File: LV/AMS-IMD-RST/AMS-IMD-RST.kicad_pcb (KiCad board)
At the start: 2 copper layers, 76.3 x 61.5 mm, 56 parts, among them J1 2P Droit 2-11-2022, J2 2P Droit 2-11-2022, J3 2P Droit 2-11-2022, J4 2P Droit 2-11-2022, J5 2P Droit 2-11-2022, J7 4P Droit 22-11-2042, K1 Relais PCB, K2 Bistable V23079B1201B301, K3 Relais PCB, K4 Bistable V23079B1201B301, Q1 NMOS SQ2348ES-T1_GE3, Q2 NMOS SQ2348ES-T1_GE3, Q3 NMOS SQ2348ES-T1_GE3, Q4 NMOS SQ2348ES-T1_GE3, Q5 NMOS SQ2348ES-T1_GE3, Q6 NMOS SQ2348ES-T1_GE3, U1 Alim LP TSR_0.5-2450

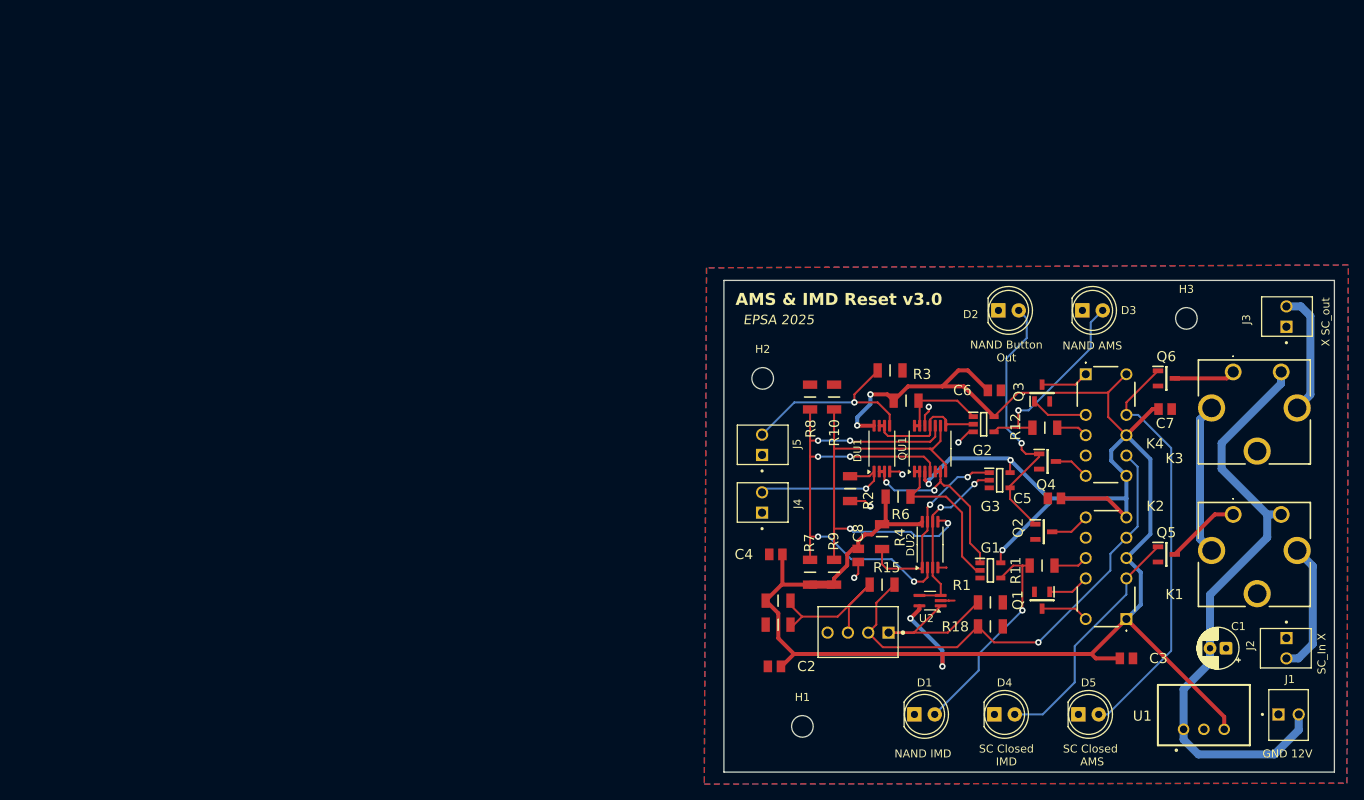
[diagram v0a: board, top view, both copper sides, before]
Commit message: Finished V1.0 of Schematic and PCB
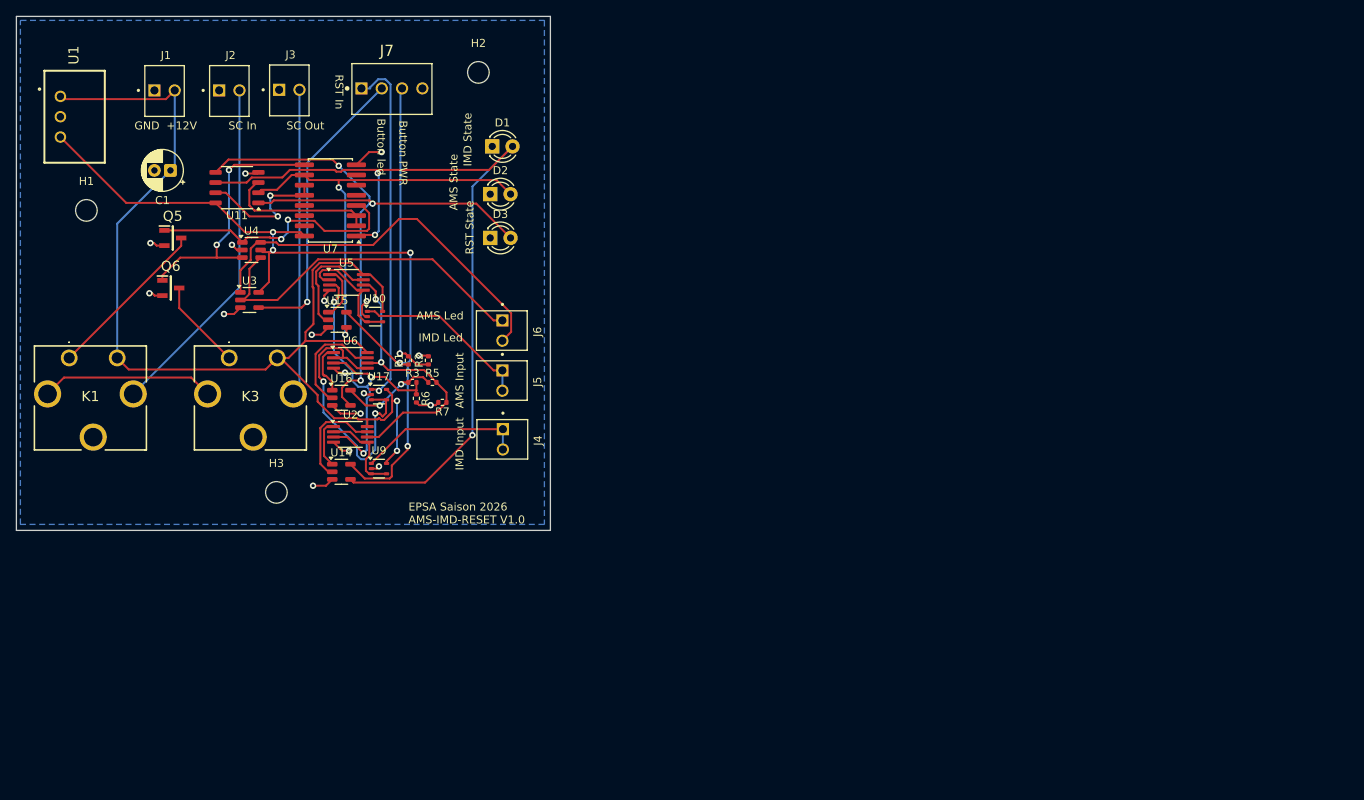
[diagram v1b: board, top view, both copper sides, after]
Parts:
- removed C2, C3, C4, C5, C6, C7, C8: 1u, EPSA_lib:CAPC2012X130N
- removed D4, D5: LED, LED_THT:LED_D5.0mm
- removed DU1, DU2: Opamp_Dual, Package_SO:TSSOP-8_4.4x3mm_P0.65mm
- removed G1, G2: Gate NAND SN74AHCT1G00DBVR, EPSA_lib:SOT95P280X145-5N
- removed G3: Gate AND SN74AHCT1G08DBVR, EPSA_lib:SOT95P280X145-5N
- removed K2, K4: Bistable V23079B1201B301, EPSA_lib:V23079B1201B301
- removed Q1, Q2, Q3, Q4: NMOS SQ2348ES-T1_GE3, EPSA_lib:SOT95P237X112-3N
- removed QU1: Opamp_Quad, Package_SO:TSSOP-14_4.4x5mm_P0.65mm
- removed R10: 82k, EPSA_lib:RESC3216X70N
- removed R11, R12: 500, EPSA_lib:RESC3216X70N
- removed R15: 3k9, EPSA_lib:RESC3216X70N
- removed R16, R17: 8k2, EPSA_lib:RESC3216X70N
- removed R18: 100k, EPSA_lib:RESC3216X70N
- removed R4: 10k, EPSA_lib:RESC3216X70N
- removed R8, R9: 12k, EPSA_lib:RESC3216X70N
- added J6: 2P Droit 2-11-2022, EPSA_lib:MOLEX_22-11-2022, F.Cu at (129.0, 73.8)
- added U10: TLV172IDCK, Package_TO_SOT_SMD:SOT-353_SC-70-5, F.Cu at (113.1, 73.3)
- added U11: 74AUC2G00, Package_SO:SSOP-8_3.9x5.05mm_P1.27mm, F.Cu at (95.8, 57.2)
- added U14: 74AHC1G08, Package_TO_SOT_SMD:SOT-23-5, F.Cu at (108.9, 92.7)
- added U15: 74AHC1G08, Package_TO_SOT_SMD:SOT-23-5, F.Cu at (108.4, 73.7)
- added U16: 74AHC1G08, Package_TO_SOT_SMD:SOT-23-5, F.Cu at (108.9, 83.4)
- added U17: TLV172IDCK, Package_TO_SOT_SMD:SOT-353_SC-70-5, F.Cu at (113.6, 83.0)
- added U3: 74AHC1G32, Package_TO_SOT_SMD:SOT-23-5, F.Cu at (97.4, 71.2)
- added U4: 74AUC2G04, Package_TO_SOT_SMD:SOT-23-6, F.Cu at (97.6, 65.0)
- added U5: MCP6562, Package_SO:MSOP-8_3x3mm_P0.65mm, F.Cu at (109.5, 69.0)
- added U6: MCP6562, Package_SO:MSOP-8_3x3mm_P0.65mm, F.Cu at (110.0, 78.8)
- added U7: 74LS279, Package_SO:SOIC-16W_5.3x10.2mm_P1.27mm, F.Cu at (107.5, 58.8)
- added U9: TLV172IDCK, Package_TO_SOT_SMD:SOT-353_SC-70-5, F.Cu at (113.6, 92.3)
- C1: value C -> 10u
- D1, D2, D3: footprint LED_THT:LED_D5.0mm -> LED_THT:LED_D3.0mm
- R1: value 500k -> 4.3k; footprint EPSA_lib:RESC3216X70N -> Resistor_SMD:R_0402_1005Metric
- R2, R3: value 500k -> 10k; footprint EPSA_lib:RESC3216X70N -> Resistor_SMD:R_0402_1005Metric
- R5: value 10k -> 4.3k; footprint EPSA_lib:RESC3216X70N -> Resistor_SMD:R_0402_1005Metric
- R6: value 10k -> 47k; footprint EPSA_lib:RESC3216X70N -> Resistor_SMD:R_0402_1005Metric
- R7: value 82k -> 10k; footprint EPSA_lib:RESC3216X70N -> Resistor_SMD:R_0402_1005Metric
- U2: value ~ -> MCP6562; footprint Package_TO_SOT_SMD:SOT-353_SC-70-5_Handsoldering -> Package_SO:MSOP-8_3x3mm_P0.65mm
- moved U1 162.7 mm to (71.8, 42.5), turned to -90 degrees
- moved J1 160.7 mm to (85.5, 45.0)
- moved J2 149.9 mm to (93.6, 45.0), turned to 0 degrees
- moved K1 146.8 mm to (74.8, 78.4)
- moved C1 144.8 mm to (87.5, 55.0)
- moved Q5 130.3 mm to (87.8, 63.5)
- moved J3 129.3 mm to (101.1, 44.9), turned to 0 degrees
- moved K3 125.5 mm to (94.8, 78.4)
- moved Q6 125.0 mm to (87.5, 69.7)
- moved H3 115.8 mm to (100.8, 95.2)
- moved H1 110.3 mm to (77.0, 60.0)
- moved J7 89.6 mm to (115.2, 44.8), turned to 0 degrees
- moved D1 88.5 mm to (127.7, 52.0)
- moved R1 78.8 mm to (117.2, 78.8), turned to 90 degrees
- moved U2 75.4 mm to (110.0, 88.0), turned to 0 degrees
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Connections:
- C1 pad 1: GND -> +12V
- C1 pad 2: +12V -> GND
- D1 pad 2: Net-(D1-A) -> /IMD_State
- D2 pad 2: Net-(D2-A) -> /AMS_State
- D3 pad 2: Net-(D3-A) -> /Button_Output_State
- J4 pad 1: GND -> /Raw_IMD_OK
- J5 pad 1: GND -> /Raw_AMS_OK
- J7 pad 2: /Button_Input -> /LED_Button
- R1 pad 1: /Raw_Button_Output -> +5V
- R1 pad 2: GND -> /Button_Input_SCS
- R2 pad 1: /Raw_IMD_OK -> /Button_Input_SCS
- R3 pad 1: /Raw_AMS_OK -> +5V
- R3 pad 2: GND -> /4V
- R5 pad 1: /AMS_SCS_Compliance -> +5V
- R5 pad 2: +5V -> /3.5V
- R6 pad 1: +5V -> /4V
- R6 pad 2: /IMD_SCS_Compliance -> GND
- R7 pad 1: /0.75V -> /3.5V
- R7 pad 2: +5V -> GND
- U2 pad 1: /Raw_Button_Output -> Net-(U14-Pad1)
- U2 pad 2: GND -> Net-(U2A--)
- U2 pad 3: /Button_Output -> /4V
- U2 pad 4: /Button_Output -> GND
- U2 pad 5: +5V -> Net-(U2A--)
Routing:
- net +5V: track 273.5 -> 122.4 mm
- net /IMD_State: track 0.00 -> 105.9 mm, vias 0 -> 3
- net /Button_Output_State: track 0.00 -> 84.6 mm, vias 0 -> 3
- net /0.75V: track 71.0 -> 0.00 mm, vias 6 -> 0
- net +12V: track 75.9 -> 139.6 mm, vias 0 -> 2
- net /Button_Input: track 60.4 -> 0.00 mm, vias 1 -> 0
- net /4.25V: track 55.1 -> 0.00 mm, vias 2 -> 0
- net /AMS_State: track 0.00 -> 54.1 mm, vias 0 -> 2
- net /IMD_Led: track 0.00 -> 49.1 mm
- net /AMS_Led: track 0.00 -> 44.4 mm
- net /4V: track 0.00 -> 44.3 mm, vias 0 -> 3
- net /LED_Button: track 0.00 -> 36.9 mm, vias 0 -> 1
- net Net-(U17--): track 0.00 -> 36.4 mm, vias 0 -> 2
- net /3.5V: track 0.00 -> 35.5 mm, vias 0 -> 2
- net Net-(D2-A): track 33.7 -> 0.00 mm, vias 1 -> 0
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- removed copper zone on F.Cu, net GND
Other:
- board size 76.3 x 61.5 mm -> 66.8 x 64.2 mm
- board text added: "+12V"
- board text added: "AMS Input"
- board text added: "AMS Led"
- board text added: "AMS State"
- board text added: "Button PWR"
- board text added: "Button led"
- board text added: "EPSA Saison 2026 AMS-IMD-RESET V1.0"
- board text added: "GND"
- board text added: "IMD Input"
- board text added: "IMD Led"
- board text added: "IMD State"
- board text added: "RST In"
- board text added: "RST State"
- board text added: "SC In"
- board text added: "SC Out"
- board text removed: "AMS & IMD Reset v3.0"
- board text removed: "EPSA 2025"
- board text removed: "GND 12V"
- board text removed: "NAND AMS"
- board text removed: "NAND Button Out"
- board text removed: "NAND IMD"
- board text removed: "SC Closed AMS"
- board text removed: "SC Closed IMD"
- board text removed: "SC_In X"
- board text removed: "X SC_out"
